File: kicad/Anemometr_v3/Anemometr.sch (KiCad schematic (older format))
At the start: 147 parts, among them J1 TxD, J10 +Z1, J11 +Z2, J12 +Z3, J13 +Z4, J14 -Z1, J15 -Z2, J16 -Z3, J17 -Z4, J18 1 TxD+, J19 2 TxD-, J2 RxD, J20 3 RxD+, J21 4-5, J22 6 RxD-, J23 7-8, J24 Conn_01x01_Female, J25 Conn_01x01_Female, J3 SCL, J4 SDA, J5 RST, J6 +EXT, J7 -EXT, J8 SWD, J9 SWC, Q1 5N10, U1 STM32F103C8Tx, U2 TS5A3166DBVR, U3 TS5A3166DBVR, U4 LMR14206, U6 NCP1117-3.3, U8 TLV3201DBV, U9 MCP1703-3.3, Y1 CSTCE8M00G52A-R0, Y2 ECS-250-20-33

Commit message: изменено:      kicad/Anemometr_v3/Anemometr-cache.lib 	изменено:      kicad/Anemometr_v3/Anemometr.kicad_pcb 	изменено:      kicad/Anemometr_v3/Anemometr.kicad_pcb-bak 	изменено:      kicad/Anemometr_v3/Anemometr.pro 	изменено:      kicad/Anemometr_v3/Anemometr.sch 	изменено:      kicad/Anemometr_v3/Anemometr.sch-bak 	изменено:      kicad/Anemometr_v3/fp-info-cache
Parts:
- removed R38: 100k, Resistor_SMD:R_0603_1608Metric, symbol Device:R
- removed R39: 3k, Resistor_SMD:R_0603_1608Metric, symbol Device:R
- removed U8: TLV3201DBV, Package_TO_SOT_SMD:SOT-23-5, symbol Comparator:MCP6566
- added C32, C5, C52, C57: 0.1uF, Capacitor_SMD:C_0402_1005Metric, symbol Device:C
- added C40: 100nF, Capacitor_SMD:C_0402_1005Metric, symbol Device:C
- added C41: 1,5nF, Capacitor_SMD:C_0402_1005Metric, symbol Device:C
- added C6: 10nF, Capacitor_SMD:C_0402_1005Metric, symbol Device:C
- added C60, C61: 10uF, Capacitor_SMD:C_0805_2012Metric, symbol Device:C
- added D19: MAX4477, Package_SO:MSOP-8_3x3mm_P0.65mm, symbol Anemometr-rescue:MAX4477-My_Library
- added D20, D21: TLV3501, Package_TO_SOT_SMD:SOT-23-6, symbol My_Library:TLV3501-2
- added J26: Conn_01x01_Female, My-library:ConnMini, symbol Connector:Conn_01x01_Female
- added R31: 20k, Resistor_SMD:R_0402_1005Metric, symbol Device:R
- added R45: 1k, Resistor_SMD:R_0402_1005Metric, symbol Device:R
- added R46, R48, R50: 100k, Resistor_SMD:R_0402_1005Metric, symbol Device:R
- added R47: 5.1k, Resistor_SMD:R_0402_1005Metric, symbol Device:R
- added R49: 10k, Resistor_SMD:R_0402_1005Metric, symbol Device:R
- added R51: 3k, Resistor_SMD:R_0402_1005Metric, symbol Device:R
- added R7, R8: 3k, Resistor_SMD:R_0603_1608Metric, symbol Device:R
- added U5, U7: TS5A3166DBVR, Package_TO_SOT_SMD:SOT-23-5, symbol Analog_Switch:TS5A3166DBVR
- added U8: MCP1703-3.3, Package_TO_SOT_SMD:SOT-23, symbol Regulator_Linear:MCP1700-3302E_SOT23
- C1, C2: footprint Capacitor_SMD:C_0805_2012Metric -> Capacitor_SMD:C_0402_1005Metric
- C42, C45, C46, C47, C48, C59: footprint Capacitor_SMD:C_0603_1608Metric -> Capacitor_SMD:C_0402_1005Metric
- C55: footprint Capacitor_SMD:C_0805_2012Metric -> Capacitor_SMD:C_0603_1608Metric
- J1, J2, J24, J25, J3, J4, J5, J8, J9: footprint My-library:SMD-CONN -> My-library:ConnMini
- R17: value 100k -> 110k
- R32, R35, R36, R37, R40, R5: footprint Resistor_SMD:R_0603_1608Metric -> Resistor_SMD:R_0402_1005Metric
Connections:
- net labels added: +3.3VP, SInput, Z1-2, Z3, Z3-4, Z4, a, swc, swd
- net labels removed: Analog, SWC, SWD, SensorInput
- wire segments 288 -> 323
- no-connect marks 31 -> 23
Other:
- moved on the sheet: C1, C10, C11, C12, C13, C14, C15, C16, C17, C18, C19, C2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

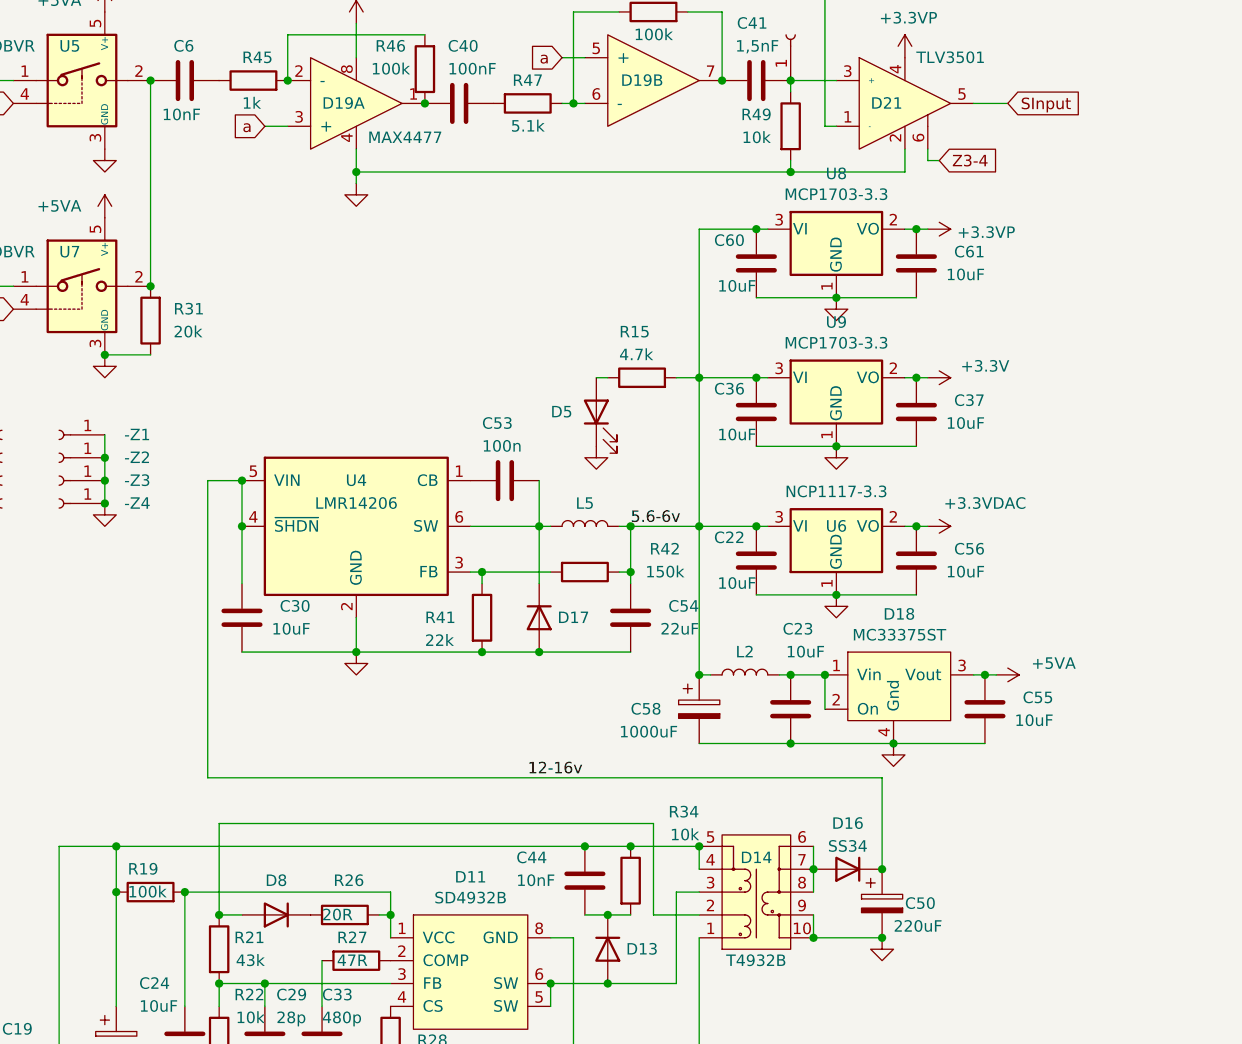
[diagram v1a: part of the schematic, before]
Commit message: изменено:      kicad/Anemometr_v3/Anemometr.kicad_pcb 	изменено:      kicad/Anemometr_v3/Anemometr.kicad_pcb-bak 	изменено:      kicad/Anemometr_v3/Anemometr.sch 	изменено:      kicad/Anemometr_v3/Anemometr.sch-bak
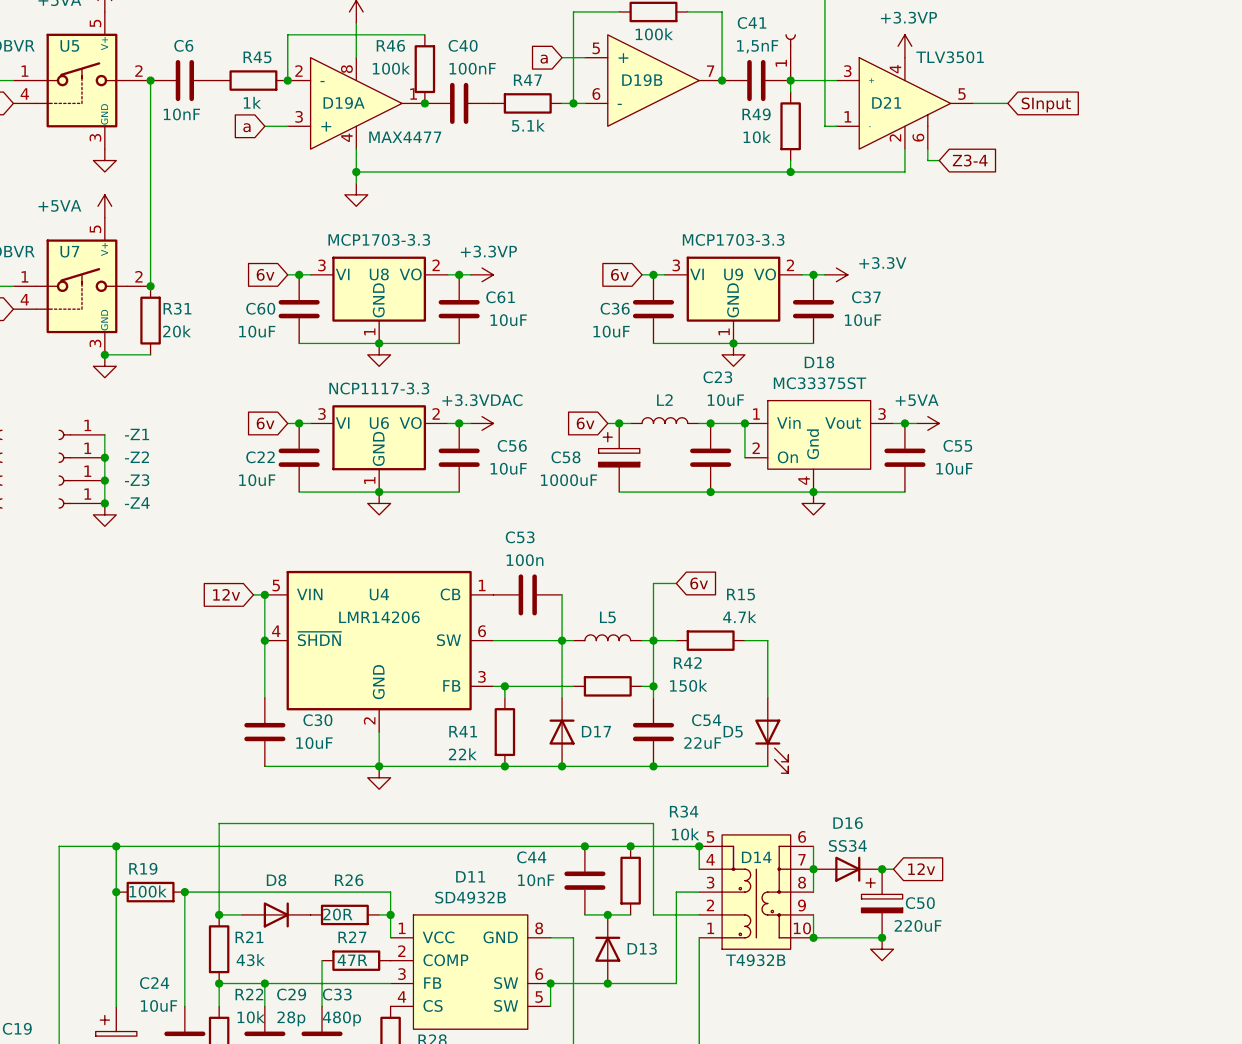
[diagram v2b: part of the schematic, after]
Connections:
- net 12-16v renamed 12v
- net 5.6-6v renamed 6v
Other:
- moved on the sheet: C22, C23, C30, C36, C37, C53, C54, C55, C56, C58, C60, C61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
